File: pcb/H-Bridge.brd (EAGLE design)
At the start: 74.6 x 86.3 mm, 49 parts, among them IC1 L293D, T1_PNP BC337, T2_NPN BC327, T3_PNP BC337, T4_NPN BC327

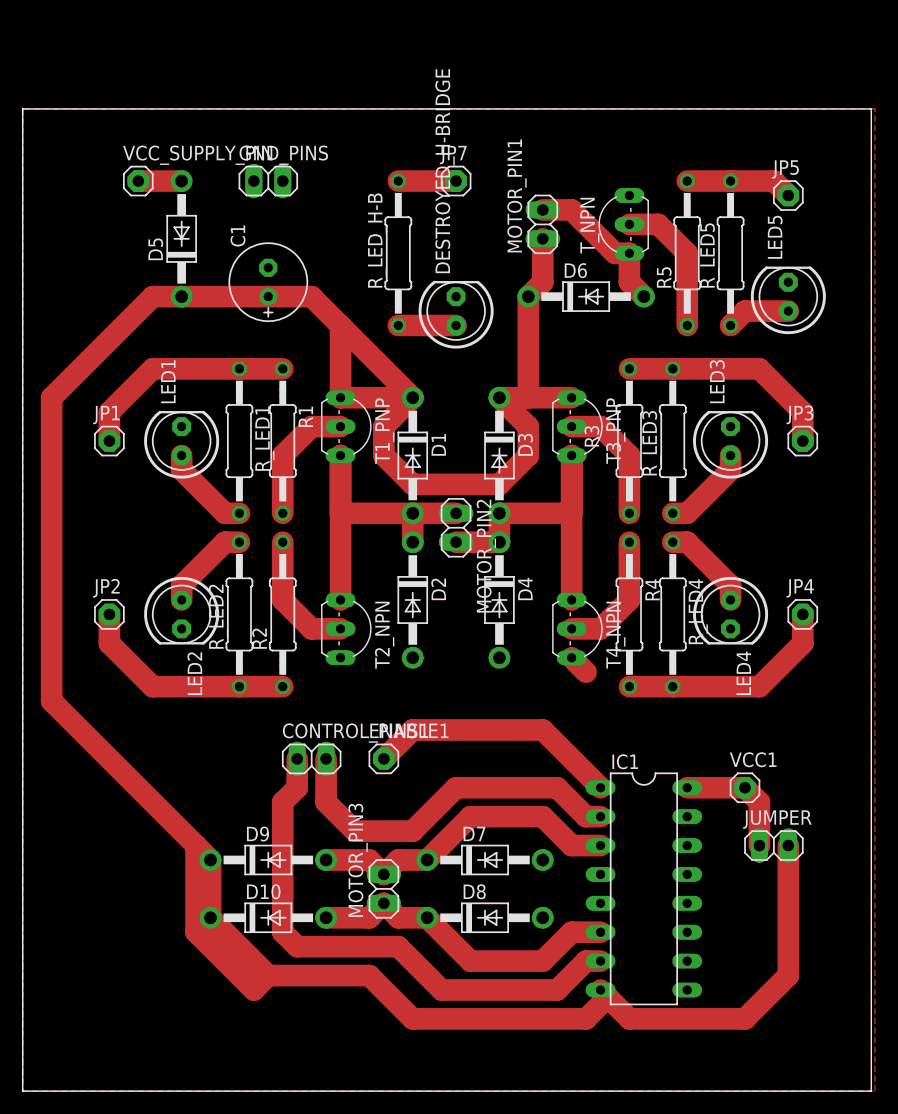
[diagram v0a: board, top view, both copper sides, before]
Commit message: Add files via upload
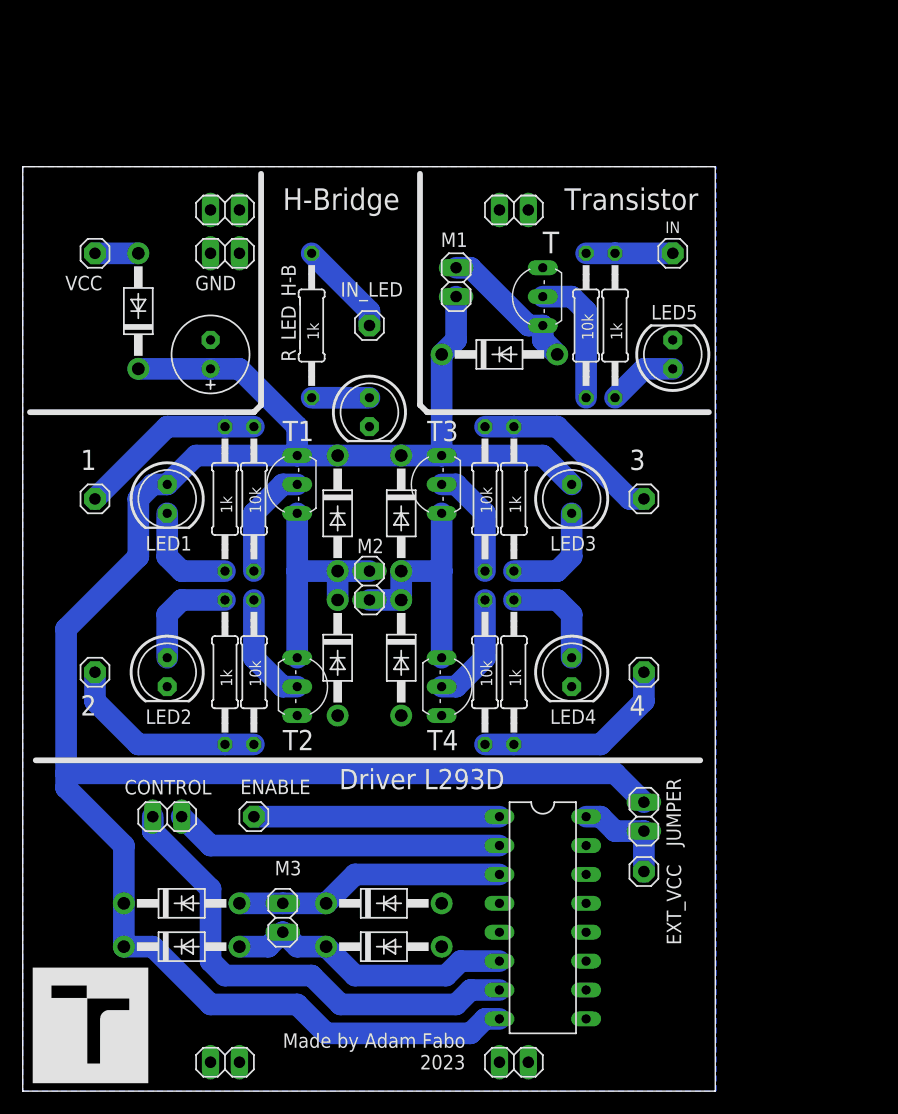
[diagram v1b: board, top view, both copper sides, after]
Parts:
- removed CONTROL_PINS1, GND_PINS, MOTOR_PIN1, MOTOR_PIN2, MOTOR_PIN3: (no value), pinhead:1X02
- removed ENABLE1, VCC1, VCC_SUPPLY_PIN: (no value), adafruit:1X01
- added BLIND-1, BLIND-2, BLIND-3, BLIND-4, CONTROL, GND, M1, M2, M3: (no value), pinhead:1X02
- added ENABLE, EXT_VCC, VCC: (no value), adafruit:1X01
- T1_PNP, T3_PNP: value BC337 -> BC237; device transistor:TO92-EBC -> transistor-neu-to92:TO92-CBE
- T2_NPN, T4_NPN, T_NPN: value BC327 -> BC337
- moved JP3 14.9 mm to (54.6, 52.1)
- moved JP4 14.9 mm to (54.6, 36.8)
- moved LED3 14.9 mm to (48.3, 52.1), turned to 270 degrees
- moved LED4 14.9 mm to (48.3, 36.8)
- moved R_LED3 14.9 mm to (43.2, 52.1)
- moved R_LED4 14.9 mm to (43.2, 36.8)
- moved JP7 14.8 mm to (30.5, 67.3)
- moved R3 13.7 mm to (40.6, 52.1)
- moved R4 13.7 mm to (40.6, 36.8)
- moved T3_PNP 13.7 mm to (36.8, 53.3), turned to 90 degrees
- moved T4_NPN 12.5 mm to (36.8, 35.6)
- moved R_LED5 12.0 mm to (52.1, 67.3)
- moved JUMPER 11.7 mm to (54.6, 24.1), turned to 90 degrees
- moved DESTROYED_H-BRIDGE 11.7 mm to (30.5, 59.7), turned to 270 degrees
- moved JP5 11.4 mm to (57.1, 73.7)
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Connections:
- net GND: now also GND.1, GND.2; no longer GND_PINS.1, GND_PINS.2, LED1.K, LED3.K
- net N$1: now also M2.1; no longer MOTOR_PIN2.1
- net N$10: now also LED3.K; no longer LED3.A
- net N$14: now also VCC.1; no longer VCC_SUPPLY_PIN.1
- net N$20: now also M3.1; no longer MOTOR_PIN3.1
- net N$22: now also M1.2; no longer MOTOR_PIN1.2
- net N$23: now also ENABLE.1; no longer ENABLE1.1
- net N$24: now also M3.2; no longer MOTOR_PIN3.2
- net N$25: now also EXT_VCC.1; no longer VCC1.1
- net N$26: now also CONTROL.1; no longer CONTROL_PINS1.1
- net N$27: now also CONTROL.2; no longer CONTROL_PINS1.2
- net N$3: now also M2.2; no longer MOTOR_PIN2.2
- net N$5: now also LED1.K; no longer LED1.A
- net VCC: now also LED1.A, LED3.A, M1.1; no longer MOTOR_PIN1.1
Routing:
- net VCC: track 237.8 -> 206.5 mm
- net N$1: track 38.1 -> 21.6 mm
- net N$3: track 38.1 -> 21.6 mm
- net N$26: track 46.9 -> 42.3 mm
- net N$24: track 27.8 -> 23.9 mm
- net N$16: track 5.08 -> 8.45 mm
- net N$2: track 19.4 -> 16.6 mm
- net N$11: track 19.4 -> 16.6 mm
- net N$27: track 31.6 -> 29.0 mm
- net N$20: track 27.8 -> 25.5 mm
- net N$18: track 9.42 -> 7.62 mm
- net GND: track 1.80 -> 0.00 mm
- net N$25: track 10.7 -> 9.16 mm
- net N$6: track 7.93 -> 9.42 mm
- net N$15: track 7.93 -> 9.42 mm
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- added copper zone on layer 16, net GND
- removed copper zone on layer 1, net GND
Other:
- board size 74.6 x 86.3 mm -> 60.9 x 81.3 mm
- board text added: "1"
- board text added: "10k"
- board text added: "1k"
- board text added: "2"
- board text added: "2023"
- board text added: "3"
- board text added: "4"
- board text added: "Driver L293D"
- board text added: "H-Bridge"
- board text added: "IN"
- board text added: "IN_LED"
- board text added: "Made by Adam Fabo"
- board text added: "T"
- board text added: "T1"
- board text added: "T2"
- board text added: "T3"
- board text added: "T4"
- board text added: "Transistor"
